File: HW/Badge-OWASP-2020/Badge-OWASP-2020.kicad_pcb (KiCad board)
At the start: 2 copper layers, 98.6 x 65.9 mm, 33 parts, among them J1 Shitty Add-Ons, J2 Battery, J3 I2C, J4 USB_B, Q1 MMBT3904, Q2 DMG3415U-7, Q3 MMBT3904, SW1 RST, SW2 BOOT, U1 ESP32-WROOM-32, U2 CH340C, U3 AP1117

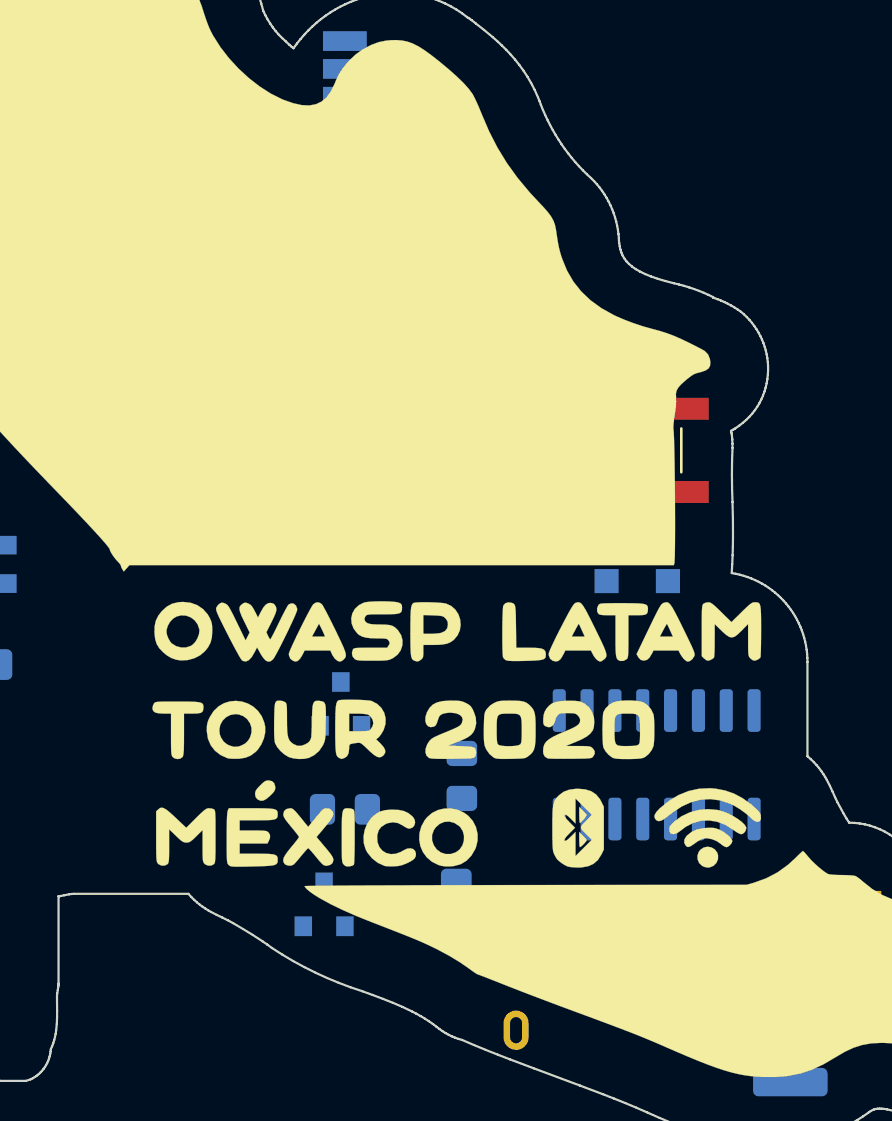
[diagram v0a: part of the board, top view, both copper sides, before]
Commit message: fix logos
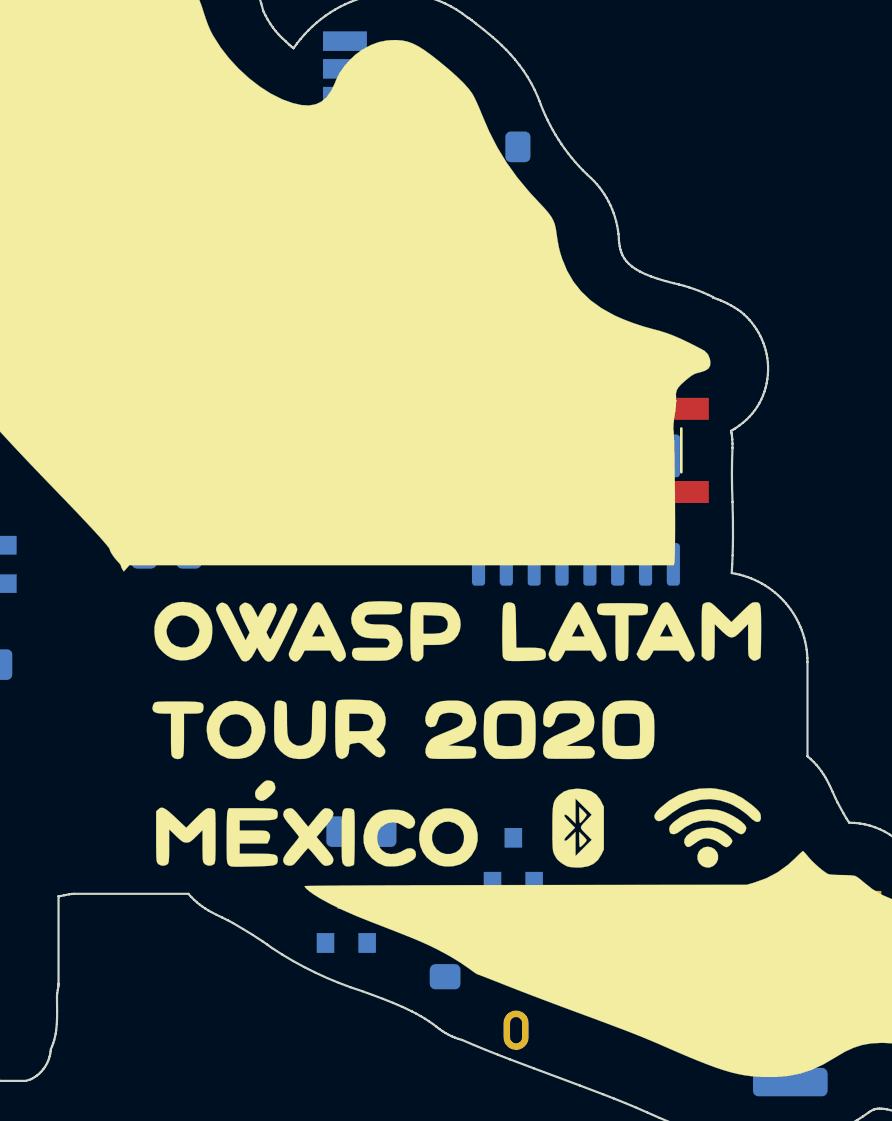
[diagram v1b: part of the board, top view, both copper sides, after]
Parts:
- moved R2 16.9 mm to (136.4, 69.1), turned to 0 degrees
- moved D3 13.4 mm to (151.8, 58.4)
- moved R1 12.6 mm to (151.4, 54.6)
- moved U2 12.2 mm to (155.1, 67.1)
- moved C1 11.6 mm to (151.4, 50.5)
- moved Q1 10.6 mm to (152.2, 83.1)
- moved G*** 5.11 mm to (145.5, 76.7)
- moved G*** 3.07 mm to (144.3, 72.1)
- moved R6 2.36 mm to (149.1, 87.4)
- moved G*** 2.05 mm to (134.9, 79.0)
- moved Q3 1.27 mm to (144.6, 85.9)
- moved R5 1.26 mm to (145.3, 81.8), turned to 180 degrees
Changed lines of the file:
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@@
-(kicad_pcb (version 20171130) (host pcbnew "(5.1.4-0-10_14)")
+(kicad_pcb (version 20171130) (host pcbnew "(5.1.4)-1")
   (general
     (thickness 1.6)
@@
     (35 F.Paste user)
     (36 B.SilkS user)
-    (37 F.SilkS user)
+    (37 F.SilkS user hide)
     (38 B.Mask user)
     (39 F.Mask user)
@@
   )
   (module Aesthetics:espressif (layer B.Cu)
-    (at 147.066 73.406 180)
+    (at 144.272 72.136 180)
     (fp_text reference G*** (at 0 0) (layer B.SilkS) hide
       (effects (font (size 1.524 1.524) (thickness 0.3)) (justify mirror))
@@
   )
   (module Aesthetics:pcbway_13x4 (layer B.Cu)
-    (at 145.034 81.788 180)
+    (at 145.542 76.708 180)
     (fp_text reference G*** (at 0 0) (layer B.SilkS) hide
       (effects (font (size 1.524 1.524) (thickness 0.3)) (justify mirror))
@@
   )
   (module Aesthetics:electronic_cats_logo_8x6 (layer B.Cu)
-    (at 135.89 77.216 180)
+    (at 134.874 78.994 180)
     (fp_text reference G*** (at 0 0) (layer B.SilkS) hide
       (effects (font (size 1.524 1.524) (thickness 0.3)) (justify mirror))
@@
   )
   (module Package_SO:SOIC-16_3.9x9.9mm_P1.27mm (layer B.Cu)
-    (at 158.75 78.74 90)
+    (at 155.067 67.121 90)
     (descr "SOIC, 16 Pin (JEDEC MS-012AC, https://www.analog.com/media/en/package-pcb-resources/package/pkg_pdf/soic_narrow-r/r_16.pdf), generated with kicad-footprint-generator ipc_gullwing_generator.py")
     (tags "SOIC SO")
@@
   )
   (module Resistor_SMD:R_0805_2012Metric_Pad1.15x1.40mm_HandSolder (layer B.Cu)
-    (at 149.606 85.081 90)
+    (at 149.098 87.385 90)
     (descr "Resistor SMD 0805 (2012 Metric), square (rectangular) end terminal, IPC_7351 nominal with elongated pad for handsoldering. (Body size source: https://docs.google.com/spreadsheets/d/1BsfQQcO9C6DZCsRaXUlFlo91Tg2WpOkGARC1WS5S8t0/edit?usp=sharing), generated with kicad-footprint-generator")
     (tags "resistor handsolder")
@@
   )
   (module Resistor_SMD:R_0805_2012Metric_Pad1.15x1.40mm_HandSolder (layer B.Cu)
-    (at 144.526 80.772)
+    (at 145.279 81.788 180)
     (descr "Resistor SMD 0805 (2012 Metric), square (rectangular) end terminal, IPC_7351 nominal with elongated pad for handsoldering. (Body size source: https://docs.google.com/spreadsheets/d/1BsfQQcO9C6DZCsRaXUlFlo91Tg2WpOkGARC1WS5S8t0/edit?usp=sharing), generated with kicad-footprint-generator")
     (tags "resistor handsolder")
@@
     (fp_line (start -1 0.6) (end 1 0.6) (layer B.Fab) (width 0.1))
     (fp_line (start -1 -0.6) (end -1 0.6) (layer B.Fab) (width 0.1))
-    (pad 2 smd roundrect (at 1.025 0) (size 1.15 1.4) (layers B.Cu B.Paste B.Mask) (roundrect_rratio 0.217391)
+    (pad 2 smd roundrect (at 1.025 0 180) (size 1.15 1.4) (layers B.Cu B.Paste B.Mask) (roundrect_rratio 0.217391)
       (net 17 /DTR))
-    (pad 1 smd roundrect (at -1.025 0) (size 1.15 1.4) (layers B.Cu B.Paste B.Mask) (roundrect_rratio 0.217391)
+    (pad 1 smd roundrect (at -1.025 0 180) (size 1.15 1.4) (layers B.Cu B.Paste B.Mask) (roundrect_rratio 0.217391)
       (net 16 "Net-(Q1-Pad1)"))
     (model ${KISYS3DMOD}/Resistor_SMD.3dshapes/R_0805_2012Metric.wrl
@@
   )
   (module Resistor_SMD:R_0805_2012Metric_Pad1.15x1.40mm_HandSolder (layer B.Cu)
-    (at 149.86 79.248 90)
+    (at 136.389 69.088)
     (descr "Resistor SMD 0805 (2012 Metric), square (rectangular) end terminal, IPC_7351 nominal with elongated pad for handsoldering. (Body size source: https://docs.google.com/spreadsheets/d/1BsfQQcO9C6DZCsRaXUlFlo91Tg2WpOkGARC1WS5S8t0/edit?usp=sharing), generated with kicad-footprint-generator")
     (tags "resistor handsolder")
     (attr smd)
-    (fp_text reference R2 (at 0 1.65 90) (layer B.SilkS)
+    (fp_text reference R2 (at 0 1.65) (layer B.SilkS)
       (effects (font (size 1 1) (thickness 0.15)) (justify mirror))
     )
-    (fp_text value 470 (at 0 -1.65 90) (layer B.Fab)
+    (fp_text value 470 (at 0 -1.65) (layer B.Fab)
       (effects (font (size 1 1) (thickness 0.15)) (justify mirror))
     )
-    (fp_text user %R (at 0 0 90) (layer B.Fab)
+    (fp_text user %R (at 0 0) (layer B.Fab)
       (effects (font (size 0.5 0.5) (thickness 0.08)) (justify mirror))
     )
@@
     (fp_line (start -1 0.6) (end 1 0.6) (layer B.Fab) (width 0.1))
     (fp_line (start -1 -0.6) (end -1 0.6) (layer B.Fab) (width 0.1))
-    (pad 2 smd roundrect (at 1.025 0 90) (size 1.15 1.4) (layers B.Cu B.Paste B.Mask) (roundrect_rratio 0.217391)
+    (pad 2 smd roundrect (at 1.025 0) (size 1.15 1.4) (layers B.Cu B.Paste B.Mask) (roundrect_rratio 0.217391)
       (net 19 "Net-(R2-Pad2)"))
-    (pad 1 smd roundrect (at -1.025 0 90) (size 1.15 1.4) (layers B.Cu B.Paste B.Mask) (roundrect_rratio 0.217391)
+    (pad 1 smd roundrect (at -1.025 0) (size 1.15 1.4) (layers B.Cu B.Paste B.Mask) (roundrect_rratio 0.217391)
       (net 5 /NP))
     (model ${KISYS3DMOD}/Resistor_SMD.3dshapes/R_0805_2012Metric.wrl
@@
   )
   (module Resistor_SMD:R_0805_2012Metric_Pad1.15x1.40mm_HandSolder (layer B.Cu)
-    (at 157.734 65.532)
+    (at 151.393 54.61)
     (descr "Resistor SMD 0805 (2012 Metric), square (rectangular) end terminal, IPC_7351 nominal with elongated pad for handsoldering. (Body size source: https://docs.google.com/spreadsheets/d/1BsfQQcO9C6DZCsRaXUlFlo91Tg2WpOkGARC1WS5S8t0/edit?usp=sharing), generated with kicad-footprint-generator")
     (tags "resistor handsolder")
@@
   )
   (module Package_TO_SOT_SMD:SOT-23 (layer B.Cu)
-    (at 143.576 85.106 90)
+    (at 144.592 85.868 90)
     (descr "SOT-23, Standard")
     (tags SOT-23)
@@
   )
   (module Package_TO_SOT_SMD:SOT-23 (layer B.Cu)
-    (at 144.338 75.962 90)
+    (at 152.212 83.074 90)
     (descr "SOT-23, Standard")
     (tags SOT-23)
@@
   )
   (module Diode_SMD:D_SOD-123F (layer B.Cu)
-    (at 157.864 70.358 180)
+    (at 151.768 58.42 180)
     (descr D_SOD-123F)
     (tags D_SOD-123F)
@@
   )
   (module Capacitor_SMD:C_0805_2012Metric_Pad1.15x1.40mm_HandSolder (layer B.Cu)
-    (at 157.471 60.452)
+    (at 151.393 50.546)
     (descr "Capacitor SMD 0805 (2012 Metric), square (rectangular) end terminal, IPC_7351 nominal with elongated pad for handsoldering. (Body size source: https://docs.google.com/spreadsheets/d/1BsfQQcO9C6DZCsRaXUlFlo91Tg2WpOkGARC1WS5S8t0/edit?usp=sharing), generated with kicad-footprint-generator")
     (tags "capacitor handsolder")
